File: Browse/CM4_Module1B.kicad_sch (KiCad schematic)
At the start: 10 parts, among them J18 179-UJ20CHC4SMTTR

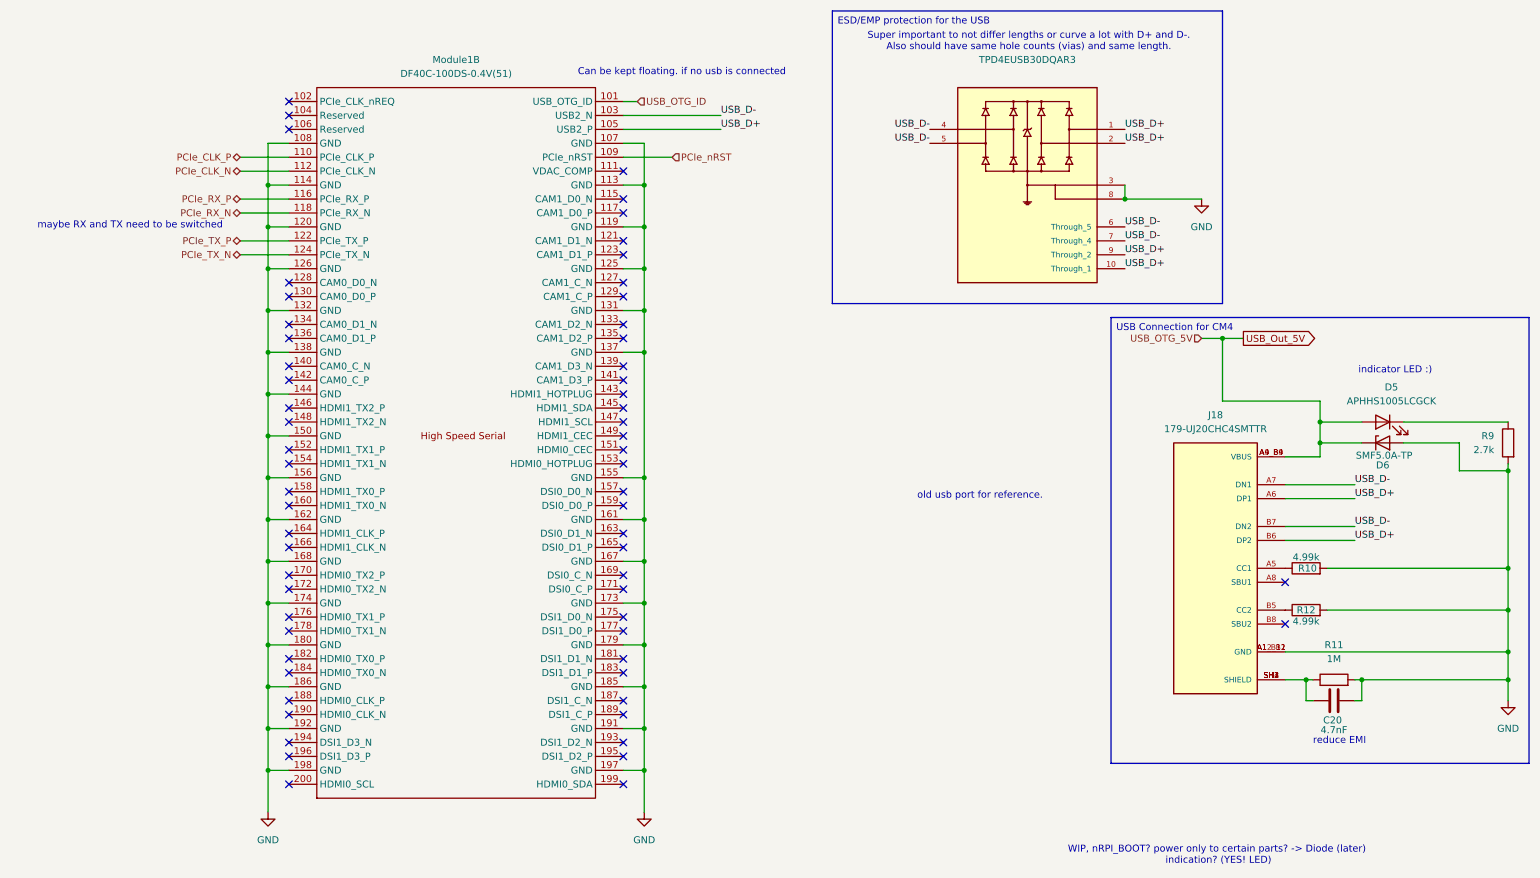
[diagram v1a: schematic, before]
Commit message: Deploying to gh-pages from @ Nautilus-UUV/nautilus-mainboard-PCB@a81f7ffbfc5f9b51f47d7f388c30fcea2673b9ea 🚀
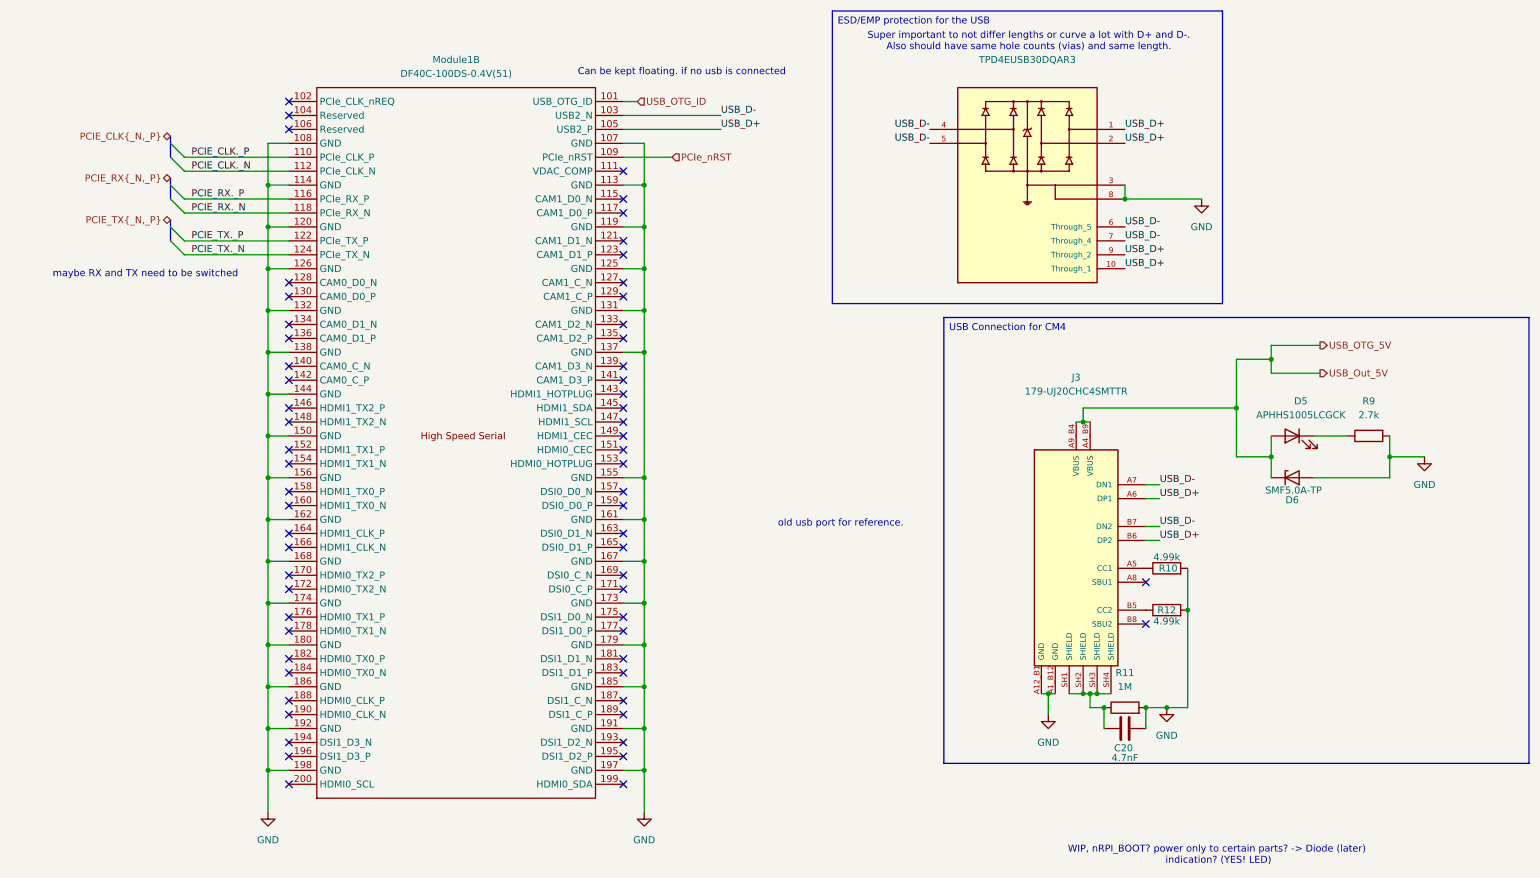
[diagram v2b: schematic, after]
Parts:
- removed J18: 179-UJ20CHC4SMTTR, dz_con:CON_Samesky_CUI_UJ20-C-H-C-4-SMT-TR, symbol #dzdb:s_con/SAME-179-UJ20CHC4SMTTR
- added J3: 179-UJ20CHC4SMTTR, dz_con:CON_Samesky_CUI_UJ20-C-H-C-4-SMT-TR, symbol #dzdb:s_con/SAME-179-UJ20CHC4SMTTR
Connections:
- net GND: now also J3.A12_B1 (GND), J3.A1_B12 (GND)
- net USB_D+: now also J3.A6 (DP1), J3.B6 (DP2)
- net USB_D-: now also J3.A7 (DN1), J3.B7 (DN2)
- net at C20.2, R11.1: now also J3.SH1 (SHIELD), J3.SH2 (SHIELD), J3.SH3 (SHIELD), J3.SH4 (SHIELD)
- net at R10.1: now also J3.A5 (CC1)
- net at R12.1: now also J3.B5 (CC2)
- net PCIe_CLK_N renamed PCIE_CLK._N
- net PCIe_CLK_P renamed PCIE_CLK._P
- net PCIe_RX_N renamed PCIE_RX._N
- net PCIe_RX_P renamed PCIE_RX._P
- net PCIe_TX_N renamed PCIE_TX._N
- net PCIe_TX_P renamed PCIE_TX._P
- net USB_Out_5V renamed USB_OTG_5V
- net USB_OTG_5V: now also J3.A4_B9 (VBUS), J3.A9_B4 (VBUS)
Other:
- note removed: "indicator LED :)"
- note removed: "reduce EMI"
- moved on the sheet: C20, D5, D6, R10, R11, R12, R9
